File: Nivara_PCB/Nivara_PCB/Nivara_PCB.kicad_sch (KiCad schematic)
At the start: 21 parts, among them CN1 ANALOG_IN, CN2 RELAY, J1 AUXILIAR, P1 NPN_IN, P2 PNP_IN, P3 D_IN, P4 RUN/STOP, P5 NPN_OUT, P6 PNP_OUT, P7 RS485, P8 ANALOG_OUT., U1 2.54-2*2, U2 FUENTE IN

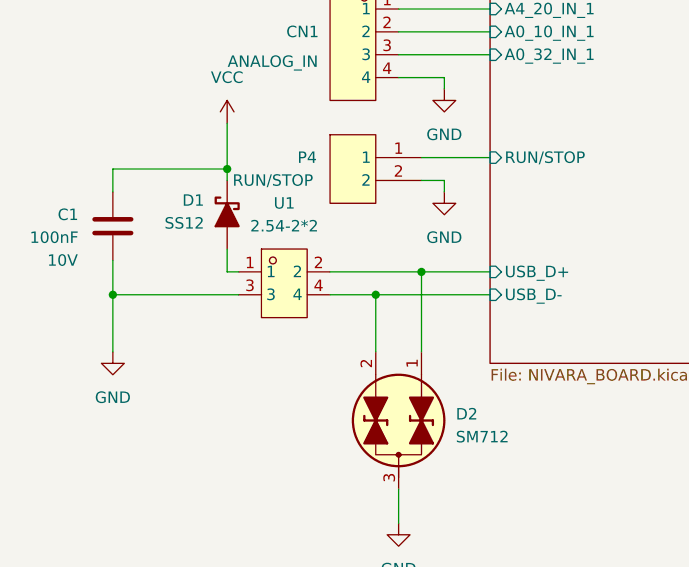
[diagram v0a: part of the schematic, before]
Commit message: Cambios en el diseño del pcb.
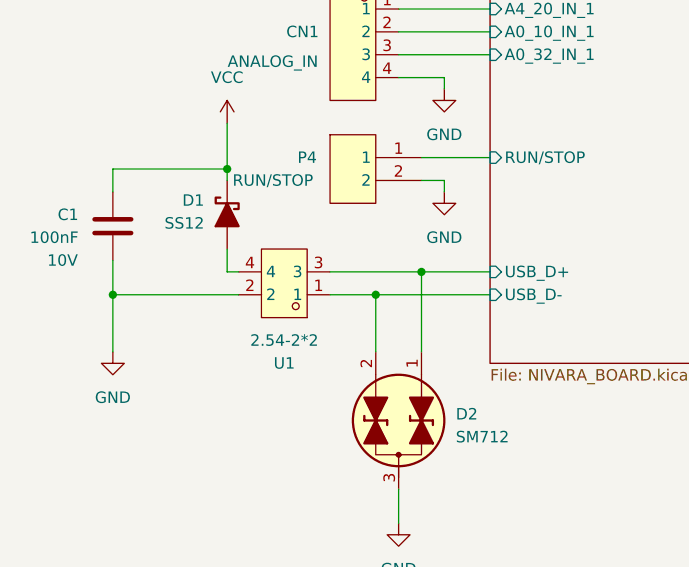
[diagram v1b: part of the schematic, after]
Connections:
- net GND: now also U1.2; no longer U1.3
- net NIVARA_BOARD/USB_D+: now also U1.3; no longer U1.2
- net NIVARA_BOARD/USB_D-: now also U1.1; no longer U1.4
- net at D1.2 (A): now also U1.4; no longer U1.1
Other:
- moved on the sheet: U1
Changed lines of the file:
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@@
 	(symbol
 		(lib_id "EasyEDA:2.54-2*2")
-		(at 50.8 120.65 0)
+		(at 50.8 120.65 180)
 		(unit 1)
 		(exclude_from_sim no)
@@
 		(on_board yes)
 		(dnp no)
-		(fields_autoplaced yes)
 		(property "Reference" "U1"
-			(at 50.8 111.76 0)
+			(at 50.8 129.54 0)
 			(effects
 				(font
@@
 		)
 		(property "Value" "2.54-2*2"
-			(at 50.8 114.3 0)
+			(at 50.8 127 0)
 			(effects
 				(font
@@
 		)
 		(property "Footprint" "Connector_PinHeader_2.54mm:PinHeader_2x02_P2.54mm_Vertical"
-			(at 50.8 129.54 0)
+			(at 50.8 111.76 0)
 			(effects
 				(font
@@
 		)
 		(property "LCSC Part" "C2977590"
-			(at 50.8 132.08 0)
+			(at 50.8 109.22 0)
 			(effects
 				(font
